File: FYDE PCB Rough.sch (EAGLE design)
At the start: 33 parts, among them CN1 USBA_FEMALE, P1 SEN-11574, T1 MMUN2133LT1G, U1 TPS61030RSAR, X1 RASPI_BOARD_B+_FP, X3 3.5mm

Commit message: updated; includes Power Booster custom library
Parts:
- removed B1: 1.8-5V, microbuilder:BATTERY
- removed C1: 10uF, microbuilder:CAP_CERAMIC0805-NOOUTLINE
- removed C2: 2.2uF, microbuilder:CAP_CERAMIC0805-NOOUTLINE
- removed C3, C6: 100uF, rcl:C-USC1210
- removed C4: 0.1uF, microbuilder:CAP_CERAMIC0805-NOOUTLINE
- removed CN1: USBA_FEMALE, microbuilder:USB_TYPEAPTHFML
- removed FID1, FID2, FID3: FIDUCIAL"", microbuilder:FIDUCIAL""
- removed JP1: (no value), adafruit:PINHD-1X6CB
- removed L1: 6.8uH, microbuilder:INDUCTOR-8X8
- removed LED1: RED, microbuilder:LED0805_NOOUTLINE
- removed LED2: GREEN, microbuilder:LED0805_NOOUTLINE
- removed R1, R3: 1.87M, microbuilder:RESISTOR_0805MP
- removed R10, R12: 49.9K 1%, microbuilder:RESISTOR0805_NOOUTLINE
- removed R11: 75K 1%, microbuilder:RESISTOR0805_NOOUTLINE
- removed R13, R4: 200K, microbuilder:RESISTOR0805_NOOUTLINE
- removed R2: 340K, microbuilder:RESISTOR_0805MP
- removed R20, R5: 1K, microbuilder:RESISTOR0805_NOOUTLINE
- removed R9: 43K 1%, microbuilder:RESISTOR0805_NOOUTLINE
- removed T1: MMUN2133LT1G, transistor:MUN2114T1-PNP_DRIVER-SC59-BEC
- removed U$10, U$11: MOUNTINGHOLE2.5, microbuilder:MOUNTINGHOLE2.5
- removed U1: TPS61030RSAR, microbuilder:VREG_TPS6103X
- removed X2: (no value), microbuilder:TERMBLOCK_1X2
- removed X3: 3.5mm, microbuilder:TERMBLOCK_1X2
- added U$1: ADAFRUITPOWERBOOSTER(FYDE), Adafruit-PowerBoost-FYDE:ADAFRUITPOWERBOOSTER(FYDE)
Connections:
- removed net 5.0V: C2.1, C3.1, C6.1, CN1.VBUS, JP1.6, R11.2, R3.2, R5.1, R9.2, U1.VOUT, X2.2
- removed net D+: CN1.D+, R11.1, R12.1
- removed net D-: CN1.D-, R10.1, R9.1
- removed net ENABLE: JP1.3, R13.2, U1.EN
- removed net GND: B1.-, C1.2, C2.2, C3.2, C4.2, C6.2, CN1.GND, JP1.2, JP1.5, LED1.C, LED2.C, R10.2, R12.2, R2.1, R4.1, U1.GND, U1.PGND, U1.SYNC, X2.1, X3.1
- removed net LBO: JP1.4, T1.B, U1.LBO
- removed net VBAT: B1.+, C1.1, C4.1, JP1.1, L1.1, R1.2, R13.1, T1.E, U1.VBAT, X3.2
- net N$1: now also U$1.5V; no longer L1.2, U1.SW
- net N$2: now also U$1.GND2; no longer LED1.A, R20.1
- net N$3: now also U$1.LBO; no longer R1.1, R2.2, U1.LBI
- net N$4: now also U$1.EN; no longer LED2.A, R5.2
- net N$5: now also U$1.GND; no longer R3.1, R4.2, U1.FB
- net N$6: now also U$1.VBAT; no longer R20.2, T1.C
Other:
- note removed: "6.8uH power w/4A current"
- note removed: "Both grounds must be connected on the PCB at only one point close to the GND pin."
- note removed: "On/Off Switch"
- note removed: "R3 = 1.9Mohm for 5.2V R3 = 1.1Mohm for 3.3V"
- note removed: "See Pg 15 1st para"

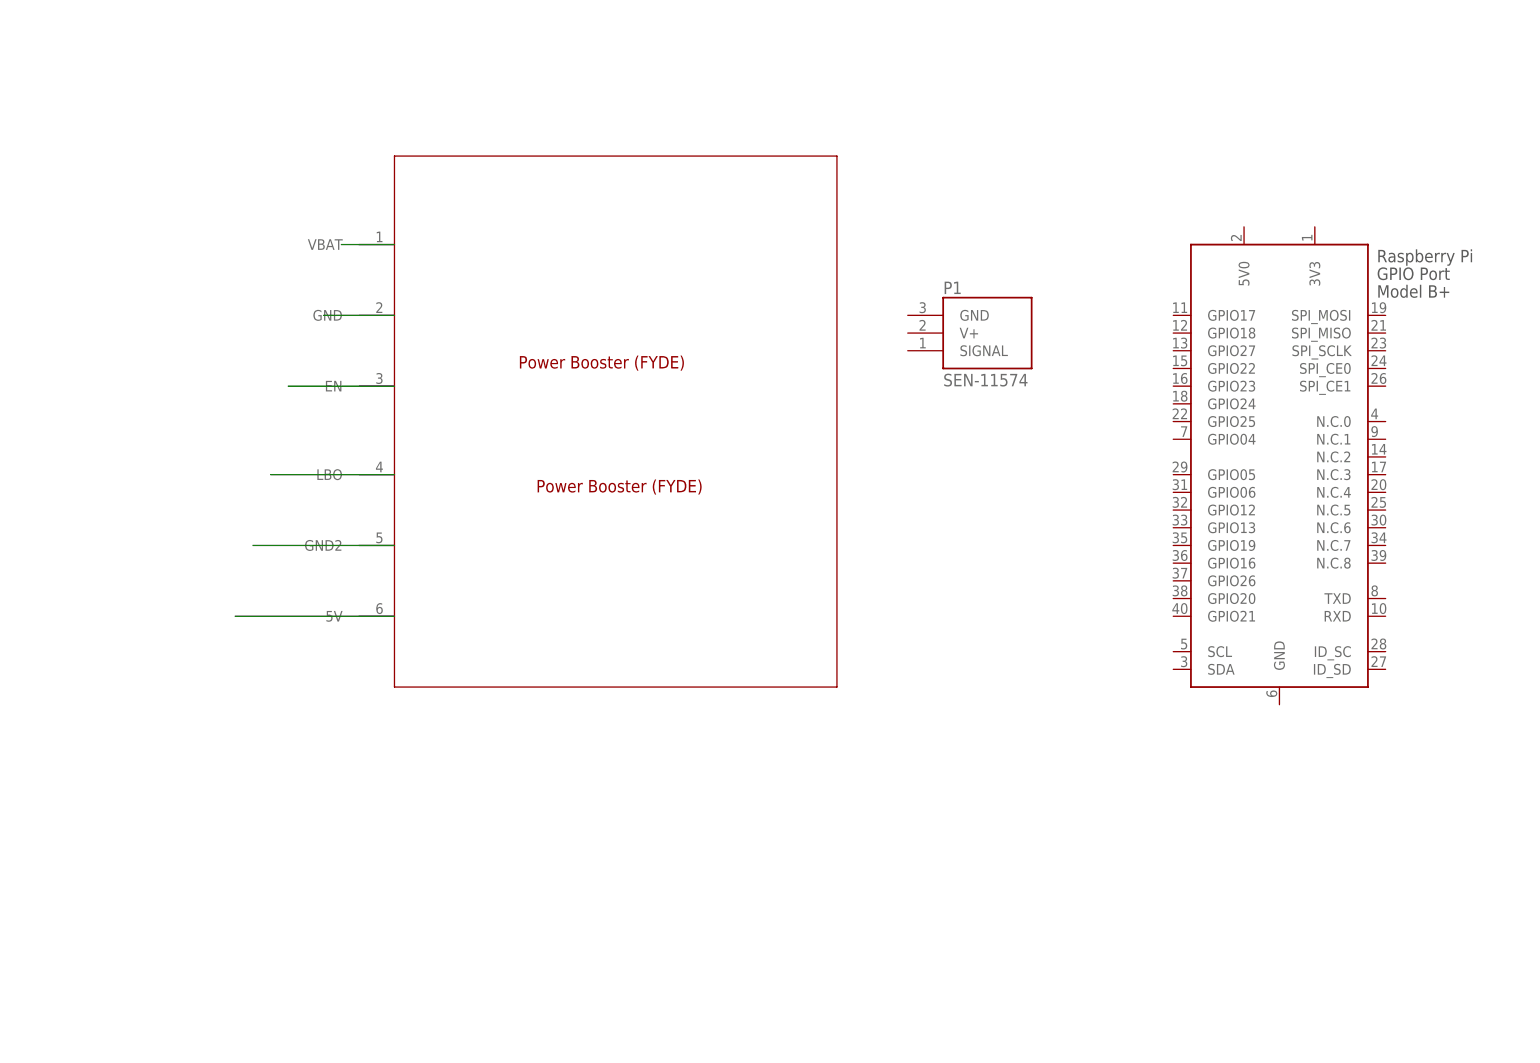
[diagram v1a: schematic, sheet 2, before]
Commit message: Add files via upload
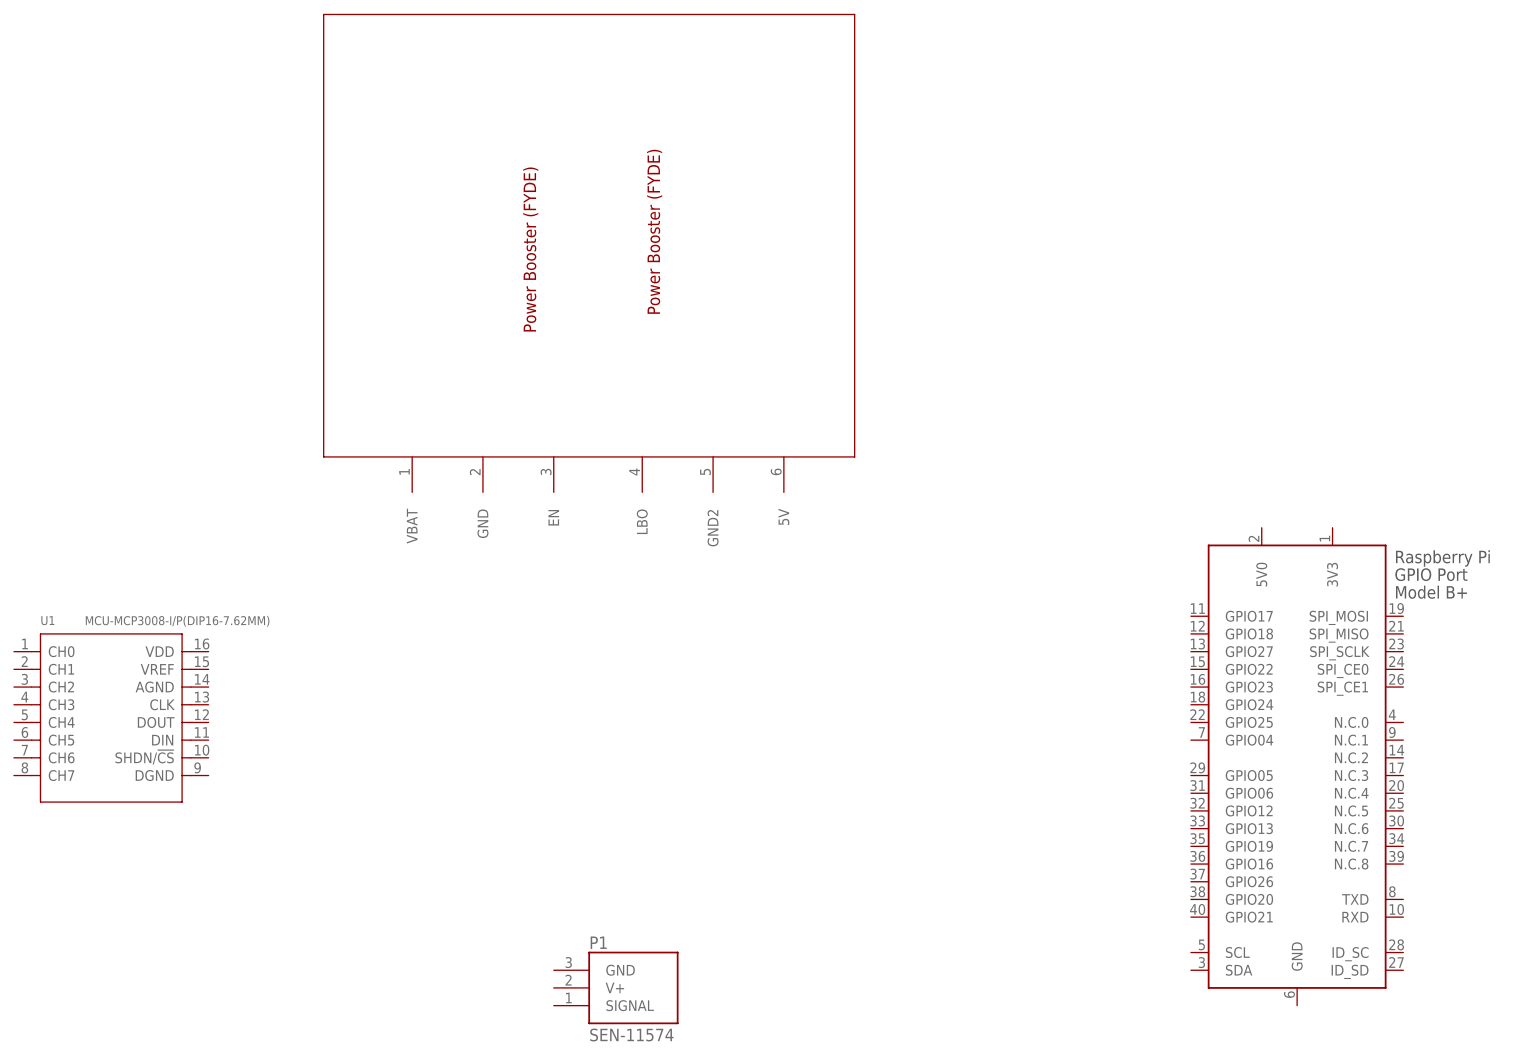
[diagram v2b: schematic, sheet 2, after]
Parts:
- added U1: MCU-MCP3008-I/P(DIP16-7.62MM), MCU-MCP3008-I_P_DIP16-7.62MM_:MCU-MCP3008-I/P(DIP16-7.62MM)
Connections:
- removed net N$1: U$1.5V
- removed net N$2: U$1.GND2
- removed net N$3: U$1.LBO
- removed net N$4: U$1.EN
- removed net N$5: U$1.GND
- removed net N$6: U$1.VBAT
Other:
- moved on the sheet: P1
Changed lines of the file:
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@@
 <part name="X1" library="raspberrypi_bastelstube_v13" deviceset="RASPI_BOARD_B+" device="_FP"/>
 <part name="U$1" library="Adafruit-PowerBoost-FYDE" deviceset="ADAFRUITPOWERBOOSTER(FYDE)" device=""/>
+<part name="U1" library="MCU-MCP3008-I_P_DIP16-7.62MM_" deviceset="MCU-MCP3008-I/P(DIP16-7.62MM)" device=""/>
 </parts>
 <sheets>
@@
 </plain>
 <instances>
-<instance part="P1" gate="G$1" x="22.86" y="160.02"/>
-<instance part="X1" gate="G$1" x="71.12" y="147.32"/>
-<instance part="U$1" gate="G$1" x="-45.72" y="109.22"/>
+<instance part="P1" gate="G$1" x="-27.94" y="66.04"/>
+<instance part="X1" gate="G$1" x="73.66" y="104.14"/>
+<instance part="U$1" gate="G$1" x="10.16" y="152.4" rot="R90"/>
+<instance part="U1" gate="G$1" x="-96.52" y="104.14"/>
 </instances>
 <busses>
 </busses>
 <nets>
-<net name="N$1" class="0">
-<segment>
-<pinref part="U$1" gate="G$1" pin="5V"/>
-<wire x1="-55.88" y1="119.38" x2="-78.74" y2="119.38" width="0.1524" layer="91"/>
-</segment>
-</net>
-<net name="N$2" class="0">
-<segment>
-<pinref part="U$1" gate="G$1" pin="GND2"/>
-<wire x1="-55.88" y1="129.54" x2="-76.2" y2="129.54" width="0.1524" layer="91"/>
-</segment>
-</net>
-<net name="N$3" class="0">
-<segment>
-<pinref part="U$1" gate="G$1" pin="LBO"/>
-<wire x1="-55.88" y1="139.7" x2="-73.66" y2="139.7" width="0.1524" layer="91"/>
-</segment>
-</net>
-<net name="N$4" class="0">
-<segment>
-<pinref part="U$1" gate="G$1" pin="EN"/>
-<wire x1="-55.88" y1="152.4" x2="-71.12" y2="152.4" width="0.1524" layer="91"/>
-</segment>
-</net>
-<net name="N$5" class="0">
-<segment>
-<pinref part="U$1" gate="G$1" pin="GND"/>
-<wire x1="-55.88" y1="162.56" x2="-66.04" y2="162.56" width="0.1524" layer="91"/>
-</segment>
-</net>
-<net name="N$6" class="0">
-<segment>
-<pinref part="U$1" gate="G$1" pin="VBAT"/>
-<wire x1="-55.88" y1="172.72" x2="-63.5" y2="172.72" width="0.1524" layer="91"/>
-</segment>
-</net>
 </nets>
 </sheet>

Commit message: schematic missing extra holes
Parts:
- X1: value RASPI_BOARD_B+_FP -> RASPI_BOARD_B+_HDC; device raspberrypi_bastelstube_v13:RASPI_BOARD_B+_FP -> raspberrypi_bastelstube_v13:RASPI_BOARD_B+_HDC
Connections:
- new net +3V3A: U1.VDD, U1.VREF, X1.3V3
- new net +5V: P1.V+, X1.5V0
- new net CLK: U1.CLK, X1.SPI_SCLK
- new net CS: U1.SHDN/!CS, X1.GPIO05
- new net GND: P1.GND, U1.AGND, U1.DGND, X1.GND
- new net MISO: U1.DOUT, X1.SPI_MISO
- new net MOSI: U1.DIN, X1.SPI_MOSI
- new net SIGNAL: P1.SIGNAL, U1.CH0
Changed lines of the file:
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@@
 <parts>
 <part name="P1" library="SEN-11574" deviceset="SEN-11574" device=""/>
-<part name="X1" library="raspberrypi_bastelstube_v13" deviceset="RASPI_BOARD_B+" device="_FP"/>
 <part name="U$1" library="Adafruit-PowerBoost-FYDE" deviceset="ADAFRUITPOWERBOOSTER(FYDE)" device=""/>
 <part name="U1" library="MCU-MCP3008-I_P_DIP16-7.62MM_" deviceset="MCU-MCP3008-I/P(DIP16-7.62MM)" device=""/>
+<part name="GND1" library="supply" deviceset="GND" device=""/>
+<part name="GND2" library="supply" deviceset="GND" device=""/>
+<part name="V1" library="supply0" deviceset="+3V3A" device=""/>
+<part name="V2" library="supply0" deviceset="+3V3A" device=""/>
+<part name="GND3" library="supply" deviceset="GND" device=""/>
+<part name="GND4" library="supply" deviceset="GND" device=""/>
+<part name="V3" library="supply0" deviceset="+5V" device=""/>
+<part name="V4" library="supply0" deviceset="+5V" device=""/>
+<part name="X1" library="raspberrypi_bastelstube_v13" deviceset="RASPI_BOARD_B+" device="_HDC"/>
 </parts>
 <sheets>
@@
 </plain>
 <instances>
+<instance part="P1" gate="G$1" x="-99.06" y="96.52"/>
+<instance part="U$1" gate="G$1" x="-50.8" y="88.9"/>
+<instance part="U1" gate="G$1" x="-101.6" y="185.42"/>
+<instance part="GND1" gate="1" x="-114.3" y="132.08"/>
+<instance part="GND2" gate="1" x="-68.58" y="187.96"/>
+<instance part="V1" gate="G$1" x="-137.16" y="177.8"/>
+<instance part="V2" gate="G$1" x="-73.66" y="200.66"/>
+<instance part="GND3" gate="1" x="-83.82" y="172.72"/>
+<instance part="GND4" gate="1" x="-109.22" y="106.68"/>
+<instance part="V3" gate="1" x="-116.84" y="99.06" rot="R90"/>
+<instance part="V4" gate="1" x="-149.86" y="177.8"/>
+<instance part="X1" gate="G$1" x="-149.86" y="142.24"/>
 </instances>
 <busses>
 </busses>
 <nets>
+<net name="GND" class="0">
+<segment>
+<pinref part="GND1" gate="1" pin="GND"/>
+<wire x1="-114.3" y1="137.16" x2="-114.3" y2="134.62" width="0.1524" layer="91"/>
+<wire x1="-127" y1="137.16" x2="-114.3" y2="137.16" width="0.1524" layer="91"/>
+<pinref part="X1" gate="G$1" pin="GND"/>
+<wire x1="-127" y1="137.16" x2="-127" y2="101.6" width="0.1524" layer="91"/>
+<wire x1="-127" y1="101.6" x2="-149.86" y2="101.6" width="0.1524" layer="91"/>
+</segment>
+<segment>
+<pinref part="U1" gate="G$1" pin="AGND"/>
+<pinref part="GND2" gate="1" pin="GND"/>
+<wire x1="-87.63" y1="190.5" x2="-68.58" y2="190.5" width="0.1524" layer="91"/>
+</segment>
+<segment>
+<pinref part="U1" gate="G$1" pin="DGND"/>
+<wire x1="-87.63" y1="177.8" x2="-83.82" y2="177.8" width="0.1524" layer="91"/>
+<pinref part="GND3" gate="1" pin="GND"/>
+<wire x1="-83.82" y1="177.8" x2="-83.82" y2="175.26" width="0.1524" layer="91"/>
+</segment>
+<segment>
+<pinref part="GND4" gate="1" pin="GND"/>
+<pinref part="P1" gate="G$1" pin="GND"/>
+<wire x1="-109.22" y1="109.22" x2="-104.14" y2="109.22" width="0.1524" layer="91"/>
+<wire x1="-104.14" y1="109.22" x2="-104.14" y2="99.06" width="0.1524" layer="91"/>
+</segment>
+</net>
+<net name="+3V3A" class="0">
+<segment>
+<pinref part="V1" gate="G$1" pin="+3V3A"/>
+<pinref part="X1" gate="G$1" pin="3V3"/>
+<wire x1="-137.16" y1="175.26" x2="-137.16" y2="170.18" width="0.1524" layer="91"/>
+<wire x1="-137.16" y1="170.18" x2="-144.78" y2="170.18" width="0.1524" layer="91"/>
+</segment>
+<segment>
+<pinref part="U1" gate="G$1" pin="VDD"/>
+<wire x1="-73.66" y1="195.58" x2="-87.63" y2="195.58" width="0.1524" layer="91"/>
+<pinref part="U1" gate="G$1" pin="VREF"/>
+<wire x1="-73.66" y1="195.58" x2="-73.66" y2="193.04" width="0.1524" layer="91"/>
+<wire x1="-73.66" y1="193.04" x2="-87.63" y2="193.04" width="0.1524" layer="91"/>
+<pinref part="V2" gate="G$1" pin="+3V3A"/>
+<wire x1="-73.66" y1="198.12" x2="-73.66" y2="195.58" width="0.1524" layer="91"/>
+<junction x="-73.66" y="195.58"/>
+</segment>
+</net>
+<net name="CLK" class="0">
+<segment>
+<pinref part="U1" gate="G$1" pin="CLK"/>
+<wire x1="-87.63" y1="187.96" x2="-83.82" y2="187.96" width="0.1524" layer="91"/>
+<label x="-83.82" y="187.96" size="1.778" layer="95" xref="yes"/>
+</segment>
+<segment>
+<wire x1="-127" y1="154.94" x2="-121.92" y2="154.94" width="0.1524" layer="91"/>
+<label x="-121.92" y="154.94" size="1.778" layer="95" xref="yes"/>
+<wire x1="-127" y1="154.94" x2="-127" y2="152.4" width="0.1524" layer="91"/>
+<pinref part="X1" gate="G$1" pin="SPI_SCLK"/>
+<wire x1="-127" y1="152.4" x2="-134.62" y2="152.4" width="0.1524" layer="91"/>
+</segment>
+</net>
+<net name="MISO" class="0">
+<segment>
+<pinref part="U1" gate="G$1" pin="DOUT"/>
+<wire x1="-87.63" y1="185.42" x2="-55.88" y2="185.42" width="0.1524" layer="91"/>
+<label x="-55.88" y="185.42" size="1.778" layer="95" xref="yes"/>
+</segment>
+<segment>
+<wire x1="-129.54" y1="157.48" x2="-111.76" y2="157.48" width="0.1524" layer="91"/>
+<label x="-111.76" y="157.48" size="1.778" layer="95" xref="yes"/>
+<wire x1="-129.54" y1="157.48" x2="-129.54" y2="154.94" width="0.1524" layer="91"/>
+<pinref part="X1" gate="G$1" pin="SPI_MISO"/>
+<wire x1="-129.54" y1="154.94" x2="-134.62" y2="154.94" width="0.1524" layer="91"/>
+</segment>
+</net>
+<net name="MOSI" class="0">
+<segment>
+<pinref part="U1" gate="G$1" pin="DIN"/>
+<wire x1="-87.63" y1="182.88" x2="-68.58" y2="182.88" width="0.1524" layer="91"/>
+<label x="-68.58" y="182.88" size="1.778" layer="95" xref="yes"/>
+</segment>
+<segment>
+<wire x1="-132.08" y1="160.02" x2="-99.06" y2="160.02" width="0.1524" layer="91"/>
+<label x="-99.06" y="160.02" size="1.778" layer="95" xref="yes"/>
+<wire x1="-132.08" y1="160.02" x2="-132.08" y2="157.48" width="0.1524" layer="91"/>
+<pinref part="X1" gate="G$1" pin="SPI_MOSI"/>
+<wire x1="-132.08" y1="157.48" x2="-134.62" y2="157.48" width="0.1524" layer="91"/>
+</segment>
+</net>
+<net name="SIGNAL" class="0">
+<segment>
+<pinref part="U1" gate="G$1" pin="CH0"/>
+<wire x1="-115.57" y1="195.58" x2="-119.38" y2="195.58" width="0.1524" layer="91"/>
+<label x="-119.38" y="195.58" size="1.778" layer="95" rot="R180" xref="yes"/>
+</segment>
+<segment>
+<pinref part="P1" gate="G$1" pin="SIGNAL"/>
+<wire x1="-104.14" y1="93.98" x2="-111.76" y2="93.98" width="0.1524" layer="91"/>
+<label x="-111.76" y="93.98" size="1.778" layer="95" rot="R180" xref="yes"/>
+</segment>
+</net>
+<net name="+5V" class="0">
+<segment>
+<pinref part="P1" gate="G$1" pin="V+"/>
+<wire x1="-104.14" y1="96.52" x2="-109.22" y2="96.52" width="0.1524" layer="91"/>
+<wire x1="-109.22" y1="96.52" x2="-109.22" y2="99.06" width="0.1524" layer="91"/>
+<wire x1="-109.22" y1="99.06" x2="-114.3" y2="99.06" width="0.1524" layer="91"/>
+<pinref part="V3" gate="1" pin="+5V"/>
+</segment>
+<segment>
+<pinref part="V4" gate="1" pin="+5V"/>
+<pinref part="X1" gate="G$1" pin="5V0"/>
+<wire x1="-149.86" y1="175.26" x2="-149.86" y2="170.18" width="0.1524" layer="91"/>
+<wire x1="-149.86" y1="170.18" x2="-154.94" y2="170.18" width="0.1524" layer="91"/>
+</segment>
+</net>
+<net name="CS" class="0">
+<segment>
+<pinref part="X1" gate="G$1" pin="GPIO05"/>
+<wire x1="-165.1" y1="134.62" x2="-170.18" y2="134.62" width="0.1524" layer="91"/>
+<label x="-170.18" y="134.62" size="1.778" layer="95" rot="R180" xref="yes"/>
+</segment>
+<segment>
+<pinref part="U1" gate="G$1" pin="SHDN/!CS"/>
+<wire x1="-87.63" y1="180.34" x2="-83.82" y2="180.34" width="0.1524" layer="91"/>
+<label x="-83.82" y="180.34" size="1.778" layer="95" xref="yes"/>
+</segment>
+</net>
 </nets>
 </sheet>
-<sheet>
-<plain>
-</plain>
-<instances>
-<instance part="P1" gate="G$1" x="-27.94" y="66.04"/>
-<instance part="X1" gate="G$1" x="73.66" y="104.14"/>
-<instance part="U$1" gate="G$1" x="10.16" y="152.4" rot="R90"/>
-<instance part="U1" gate="G$1" x="-96.52" y="104.14"/>
-</instances>
-<busses>
-</busses>
-<nets>
-</nets>
-</sheet>
